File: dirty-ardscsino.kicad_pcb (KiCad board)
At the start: 2 copper layers, 70.9 x 82 mm, 20 parts, among them J1 SCSI, J2 171825-4 (Ext. Power), J3 DM3AT-SF-PEJM5, U1 STM32 Bluepill, U2 microSD-Breakout

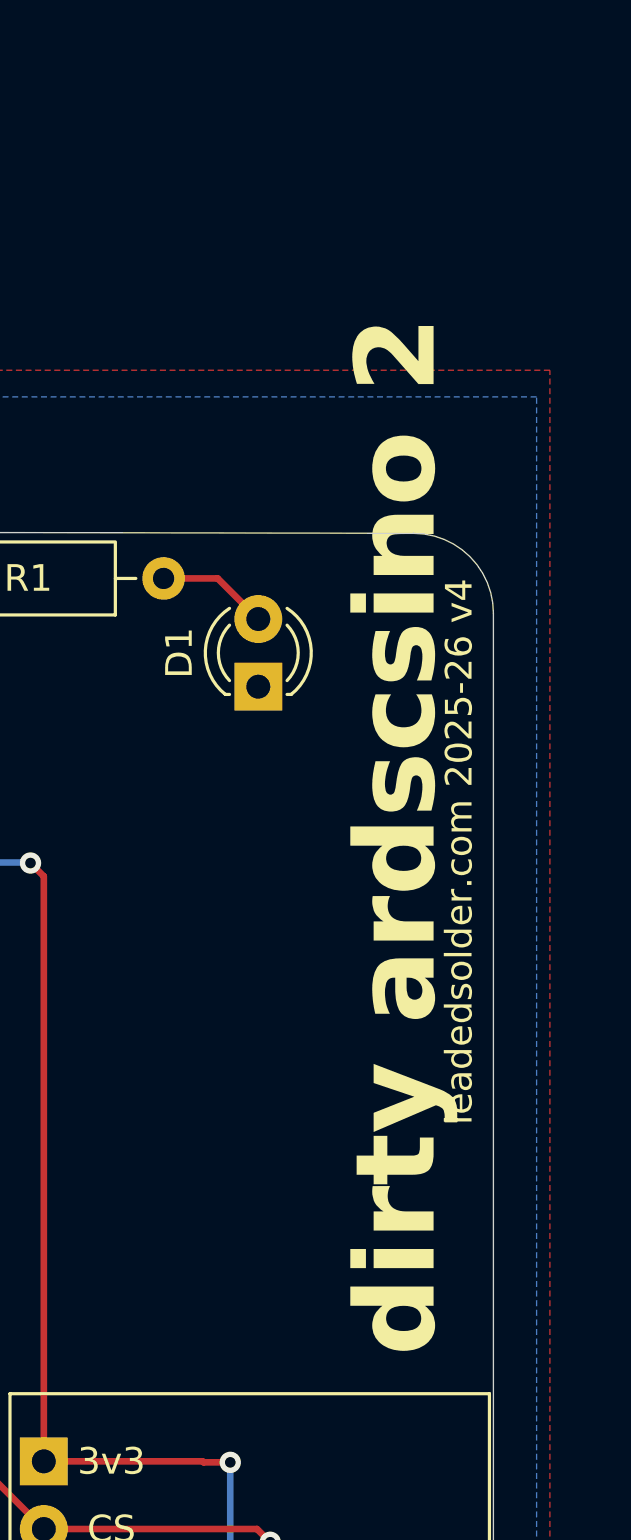
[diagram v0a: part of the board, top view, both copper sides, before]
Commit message: Touch up logo
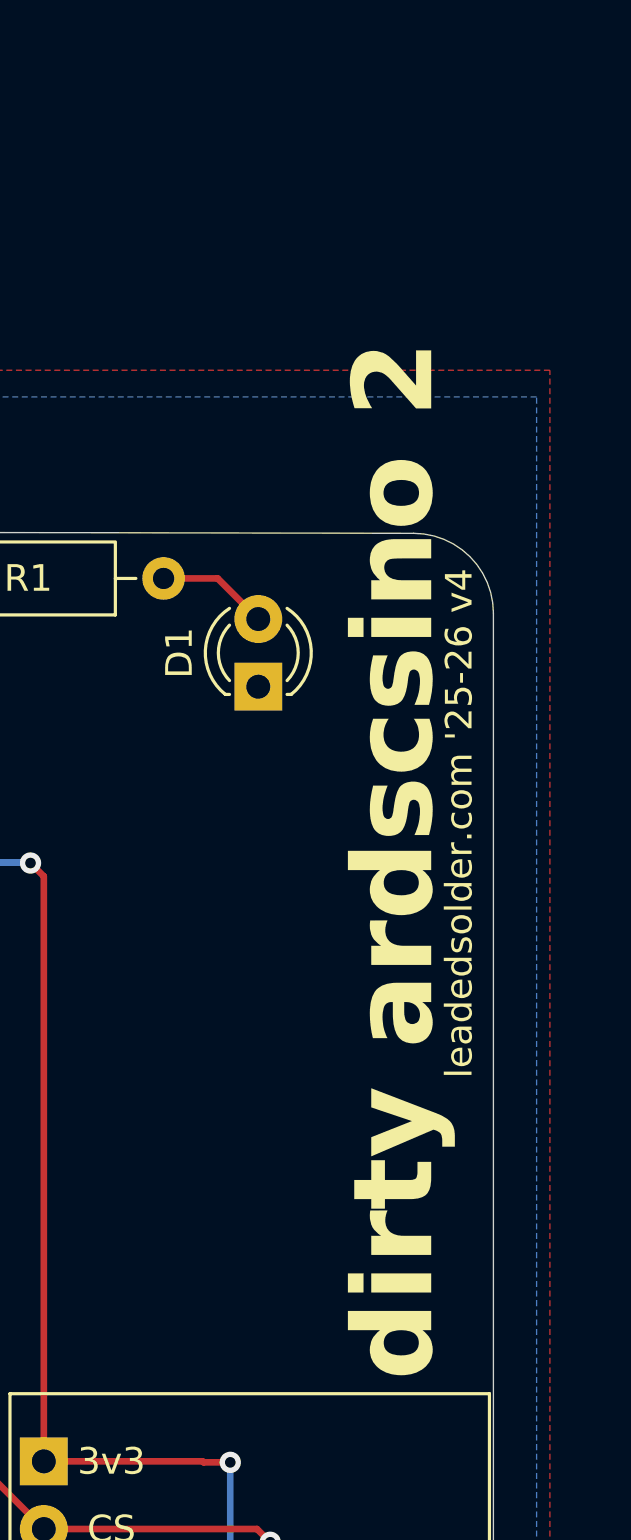
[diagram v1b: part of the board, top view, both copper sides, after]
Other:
- board text added: "leadedsolder.com '25-26 v4"
- board text removed: "leadedsolder.com 2025-26 v4"
